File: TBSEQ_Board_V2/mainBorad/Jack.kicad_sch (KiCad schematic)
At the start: 8 parts

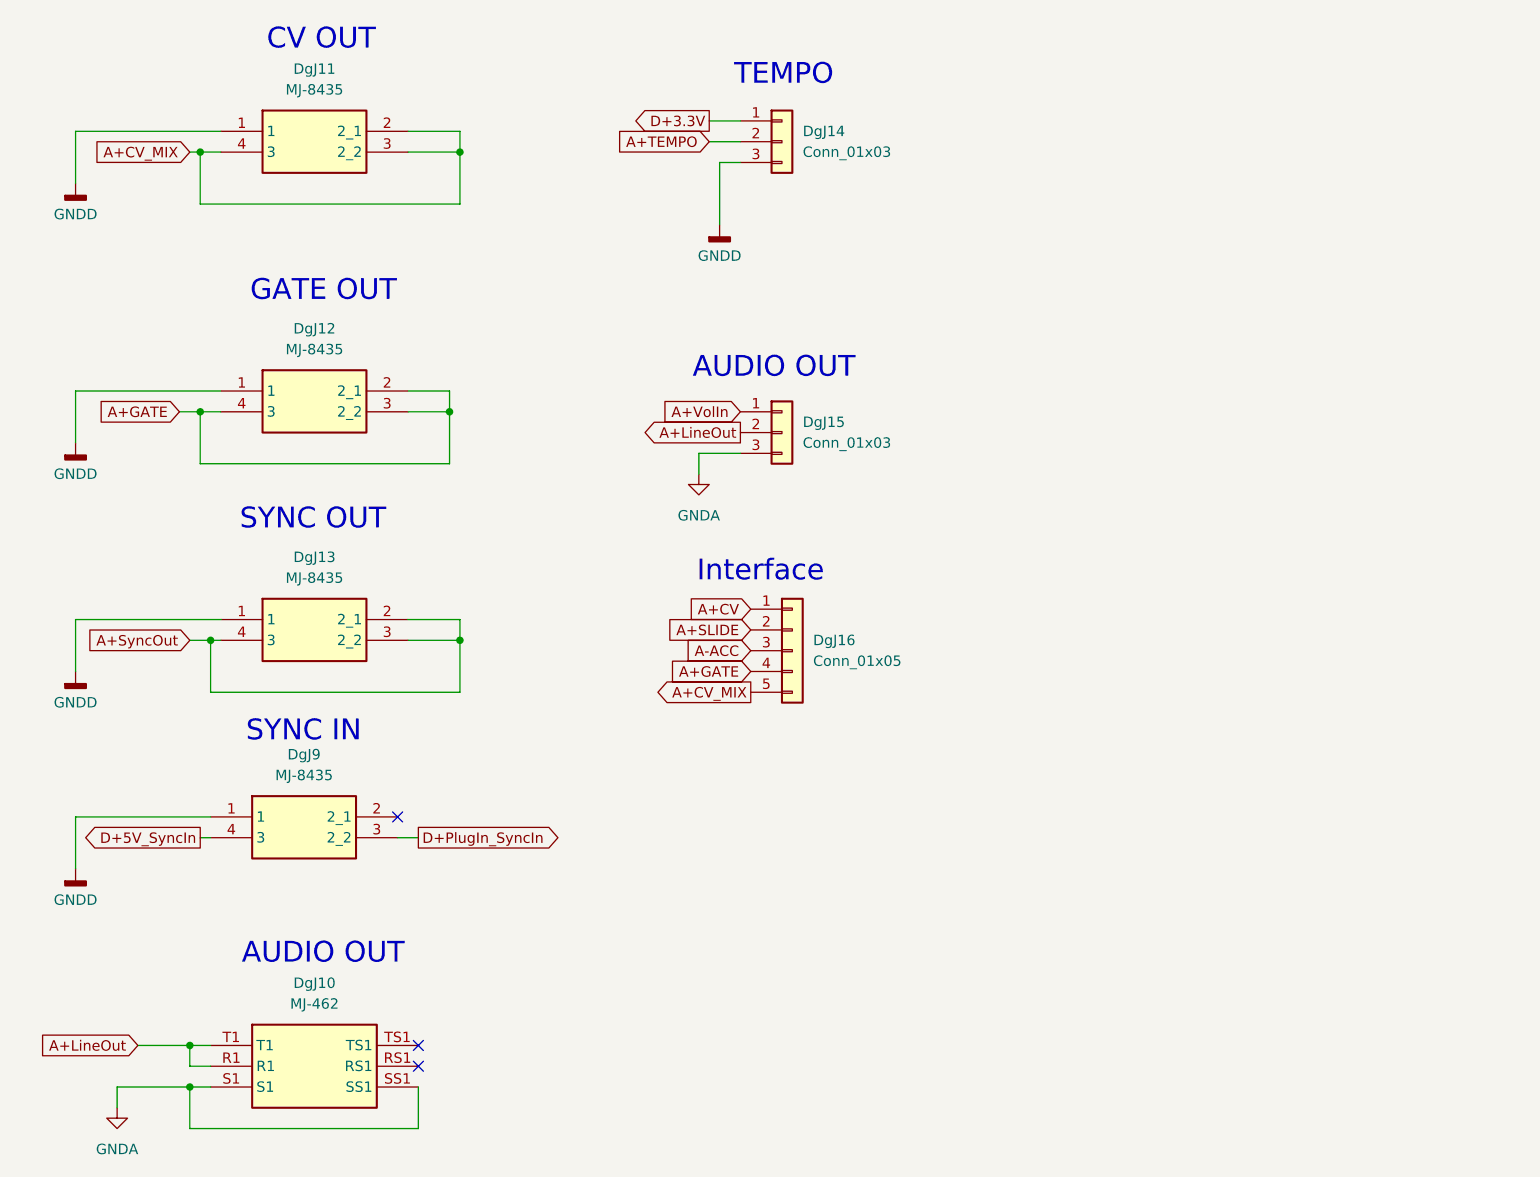
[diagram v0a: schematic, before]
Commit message: mainboard
PWS,Digi
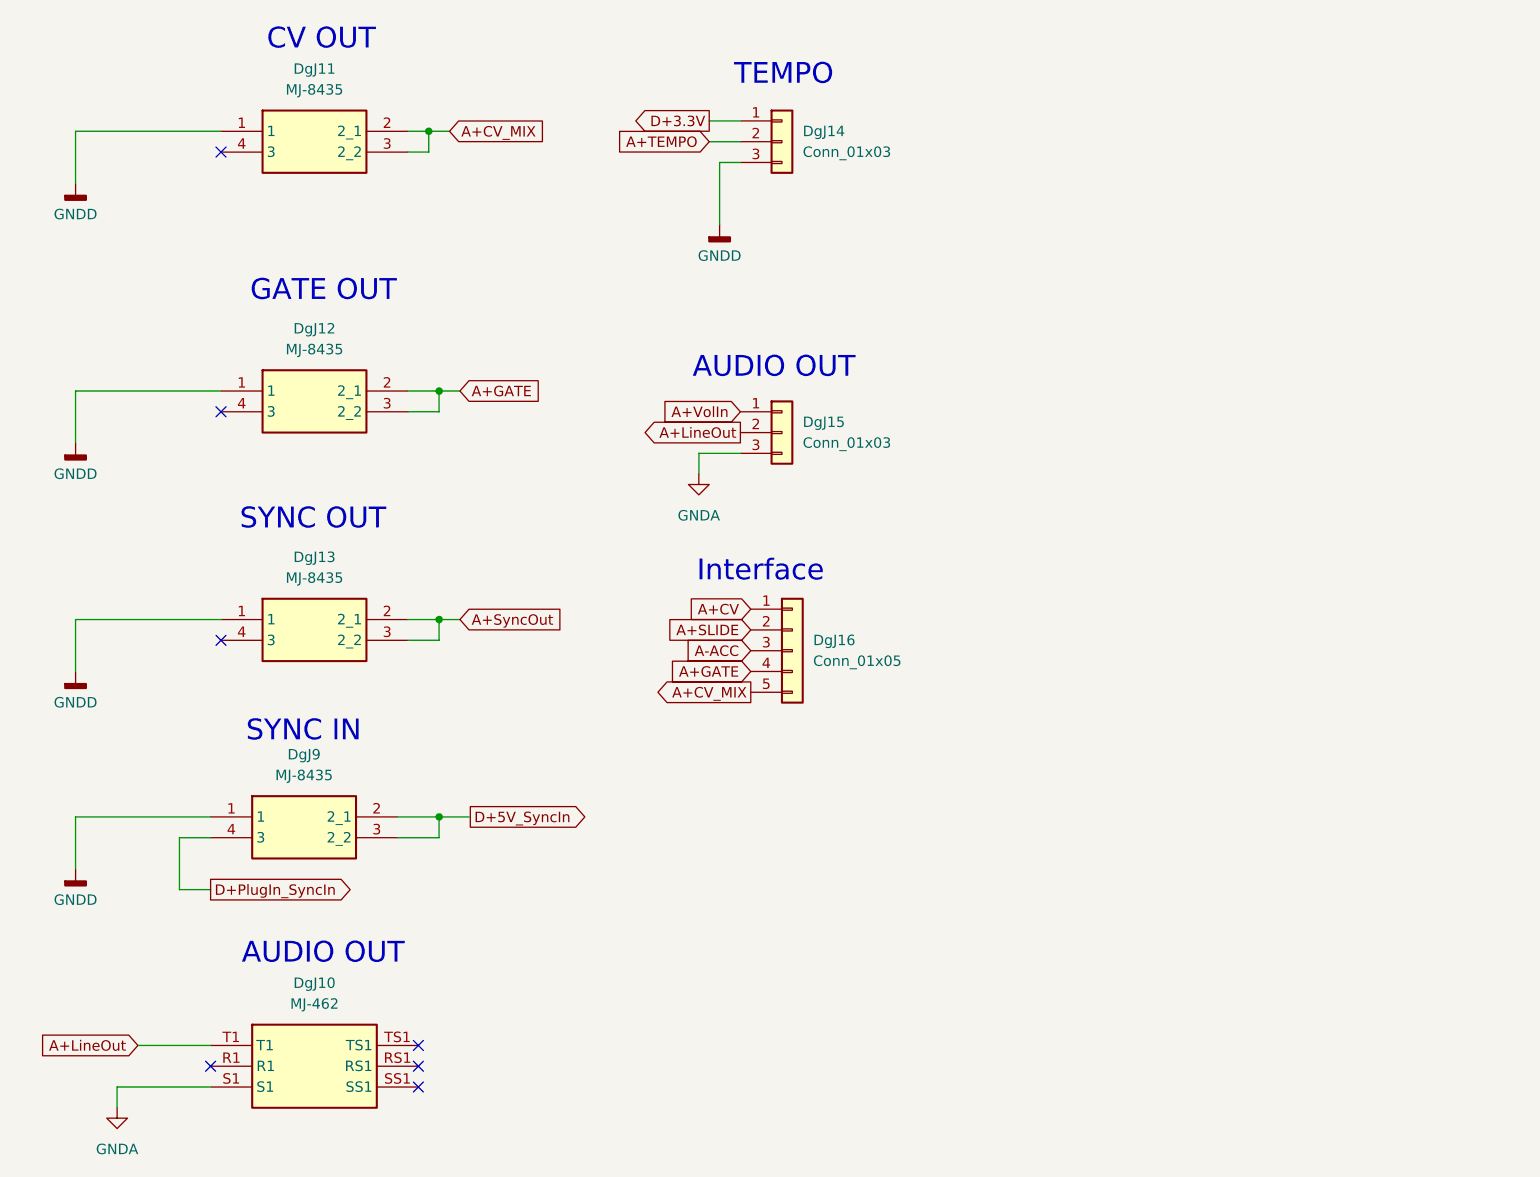
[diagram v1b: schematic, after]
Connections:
- net A+CV_MIX: no longer DgJ11.4 (3)
- net A+GATE: no longer DgJ12.4 (3)
- net A+LineOut: no longer DgJ10.R1
- net A+SyncOut: no longer DgJ13.4 (3)
- net D+5V_SyncIn: now also DgJ9.2 (2_1), DgJ9.3 (2_2); no longer DgJ9.4 (3)
- net D+PlugIn_SyncIn: now also DgJ9.4 (3); no longer DgJ9.3 (2_2)
- net GNDA: no longer DgJ10.SS1
- no-connect marks 3 -> 7

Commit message: mainBoard
AnInterface
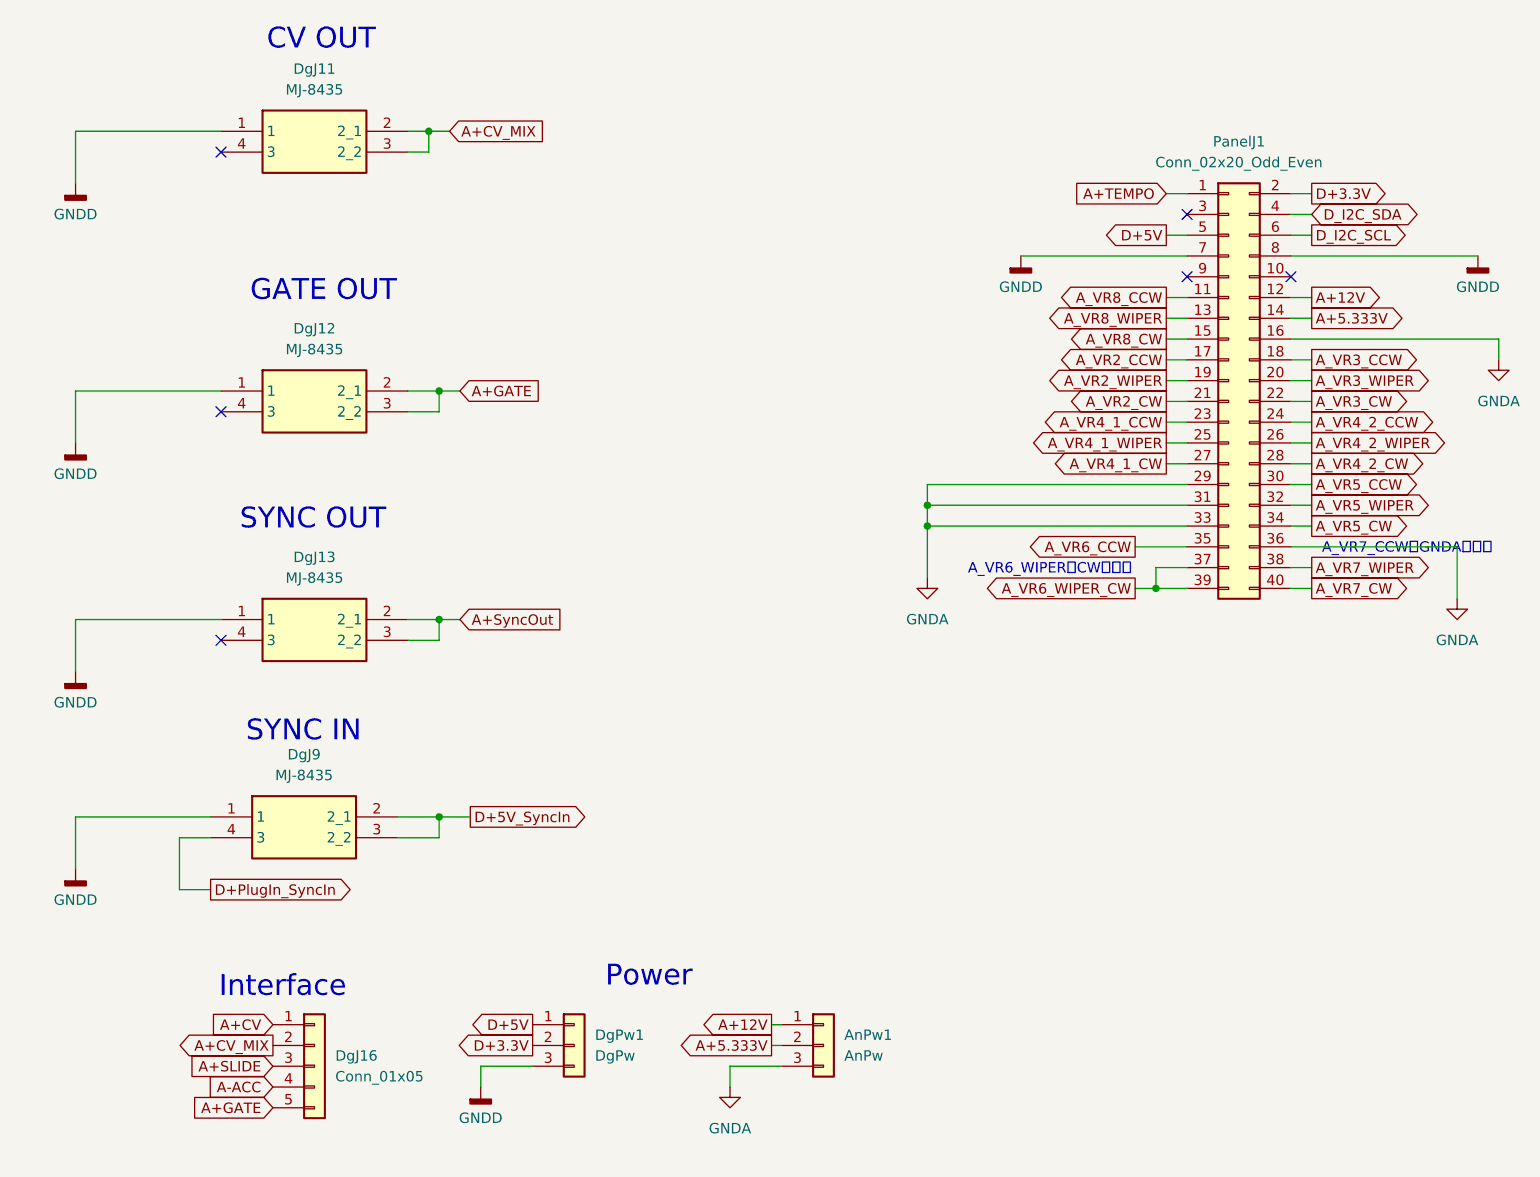
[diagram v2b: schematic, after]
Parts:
- removed DgJ10: MJ-462, MJ462, symbol SamacSys_Parts:MJ-462
- removed DgJ14, DgJ15: Conn_01x03, Connector_PinHeader_2.54mm:PinHeader_1x03_P2.54mm_Vertical, symbol Connector_Generic:Conn_01x03
- added AnPw1: AnPw, Connector_PinSocket_2.54mm:PinSocket_1x03_P2.54mm_Vertical, symbol Connector_Generic:Conn_01x03
- added DgPw1: DgPw, Connector_PinSocket_2.54mm:PinSocket_1x03_P2.54mm_Vertical, symbol Connector_Generic:Conn_01x03
- added PanelJ1: Conn_02x20_Odd_Even, Connector_PinSocket_2.54mm:PinSocket_2x20_P2.54mm_Vertical, symbol Connector_Generic:Conn_02x20_Odd_Even
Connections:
- net A+CV_MIX: now also DgJ16.2 (Pin_2); no longer DgJ16.5 (Pin_5)
- net A+GATE: now also DgJ16.5 (Pin_5); no longer DgJ16.4 (Pin_4)
- net A+SLIDE: now also DgJ16.3 (Pin_3); no longer DgJ16.2 (Pin_2)
- net A+TEMPO: now also PanelJ1.1 (Pin_1)
- net A-ACC: now also DgJ16.4 (Pin_4); no longer DgJ16.3 (Pin_3)
- net D+3.3V: now also DgPw1.2 (Pin_2), PanelJ1.2 (Pin_2)
- net GNDA: now also AnPw1.3 (Pin_3), PanelJ1.16 (Pin_16), PanelJ1.29 (Pin_29), PanelJ1.31 (Pin_31), PanelJ1.33 (Pin_33), PanelJ1.36 (Pin_36)
- net GNDD: now also DgPw1.3 (Pin_3), PanelJ1.7 (Pin_7), PanelJ1.8 (Pin_8)
- new net A+12V: AnPw1.1 (Pin_1), PanelJ1.12 (Pin_12)
- new net A+5.333V: AnPw1.2 (Pin_2), PanelJ1.14 (Pin_14)
- new net A_VR2_CCW: PanelJ1.17 (Pin_17)
- new net A_VR2_CW: PanelJ1.21 (Pin_21)
- new net A_VR2_WIPER: PanelJ1.19 (Pin_19)
- new net A_VR3_CCW: PanelJ1.18 (Pin_18)
- new net A_VR3_CW: PanelJ1.22 (Pin_22)
- new net A_VR3_WIPER: PanelJ1.20 (Pin_20)
- new net A_VR4_1_CCW: PanelJ1.23 (Pin_23)
- new net A_VR4_1_CW: PanelJ1.27 (Pin_27)
- new net A_VR4_1_WIPER: PanelJ1.25 (Pin_25)
- new net A_VR4_2_CCW: PanelJ1.24 (Pin_24)
- new net A_VR4_2_CW: PanelJ1.28 (Pin_28)
- new net A_VR4_2_WIPER: PanelJ1.26 (Pin_26)
- new net A_VR5_CCW: PanelJ1.30 (Pin_30)
- new net A_VR5_CW: PanelJ1.34 (Pin_34)
- new net A_VR5_WIPER: PanelJ1.32 (Pin_32)
- new net A_VR6_CCW: PanelJ1.35 (Pin_35)
- new net A_VR6_WIPER_CW: PanelJ1.37 (Pin_37), PanelJ1.39 (Pin_39)
- new net A_VR7_CW: PanelJ1.40 (Pin_40)
- new net A_VR7_WIPER: PanelJ1.38 (Pin_38)
- new net A_VR8_CCW: PanelJ1.11 (Pin_11)
- new net A_VR8_CW: PanelJ1.15 (Pin_15)
- new net A_VR8_WIPER: PanelJ1.13 (Pin_13)
- new net D+5V: DgPw1.1 (Pin_1), PanelJ1.5 (Pin_5)
- new net D_I2C_SCL: PanelJ1.6 (Pin_6)
- new net D_I2C_SDA: PanelJ1.4 (Pin_4)
- no-connect marks 7 -> 6
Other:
- note added: "A_VR6_WIPERはCWと接続"
- note added: "A_VR7_CCWはGNDAと接続"
- note added: "Power"
- note removed: "AUDIO OUT"
- note removed: "TEMPO"
- moved on the sheet: DgJ16
